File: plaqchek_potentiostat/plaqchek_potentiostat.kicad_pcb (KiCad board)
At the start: 4 copper layers, 46 x 59 mm, 63 parts, among them J1 Conn_01x03, J2 Conn_01x03, J3 Conn_01x02, SW2 SW_SPDT, U1 TL082, U3 TL082, U4 TL082, U5 TPS7A2050PDBVR, U6 MC79M05_TO252

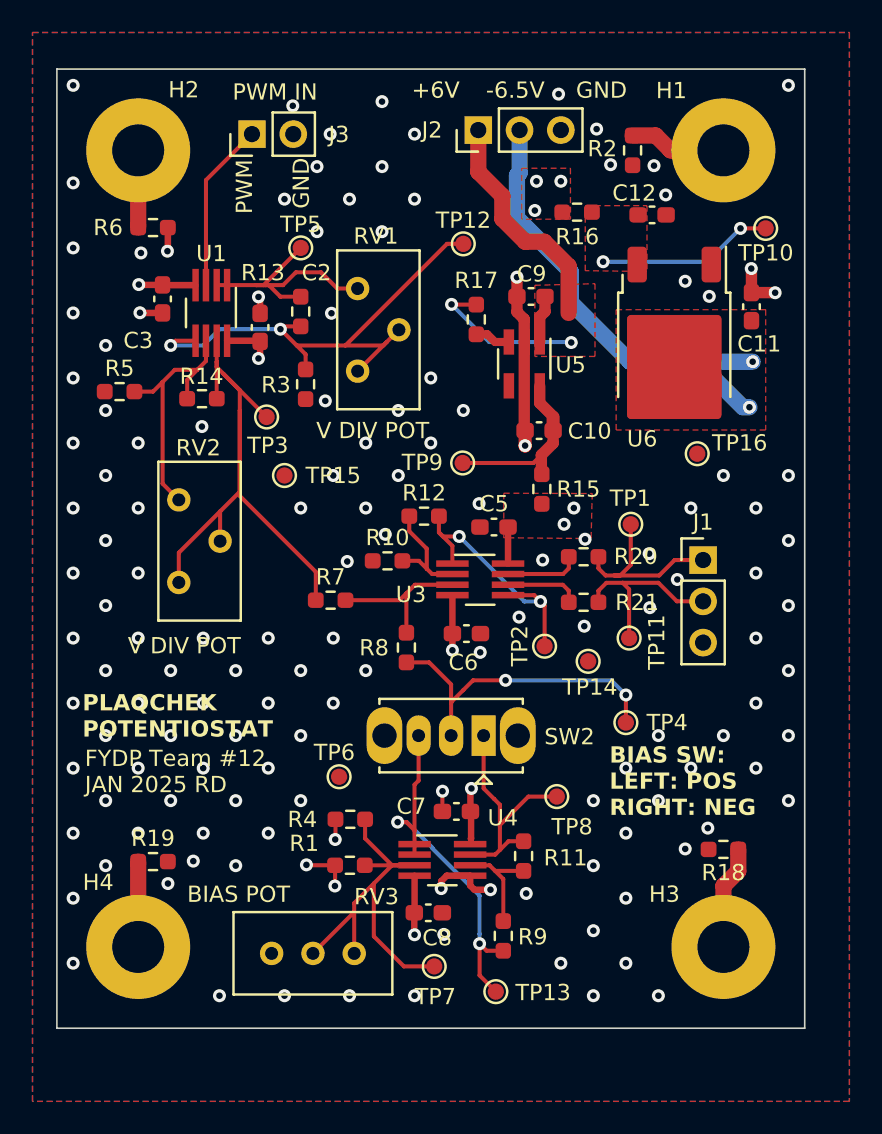
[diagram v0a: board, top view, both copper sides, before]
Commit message: finish all pcbs, generate gerber files
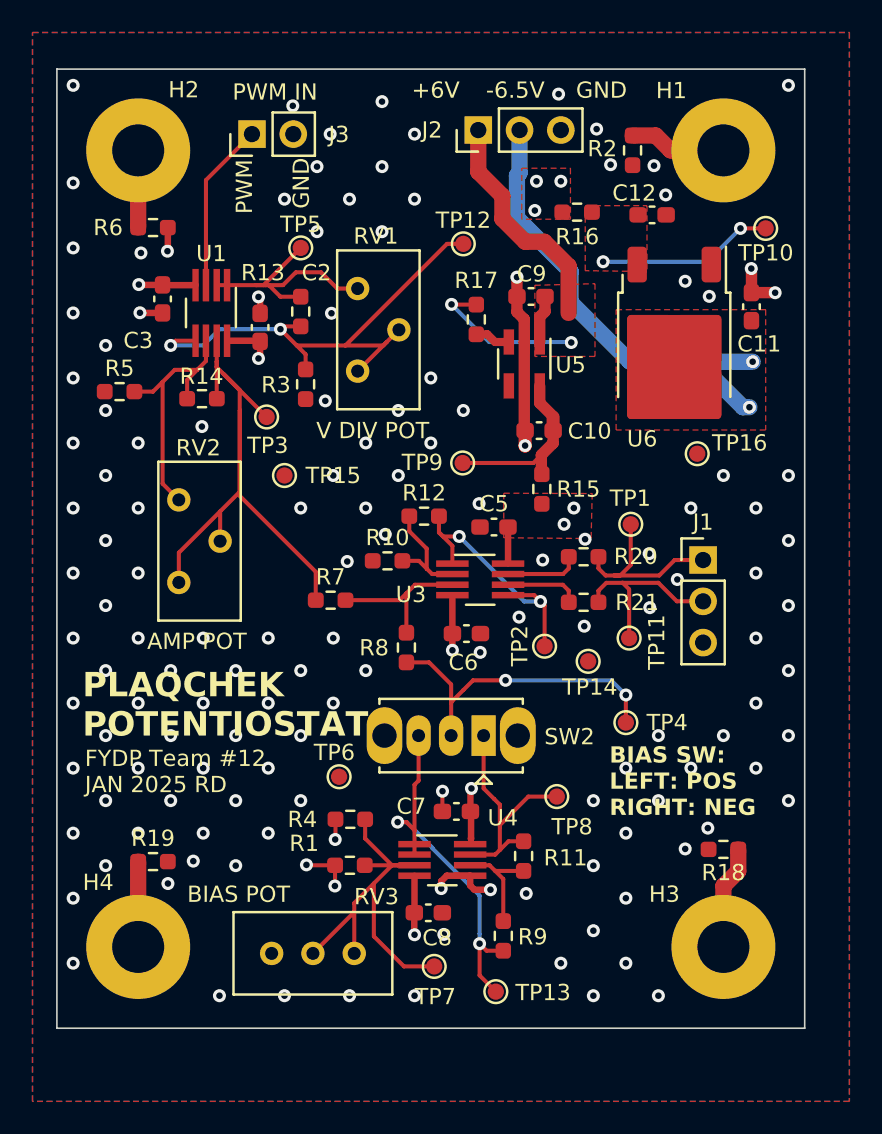
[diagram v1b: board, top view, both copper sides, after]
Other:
- board text added: "AMP POT"
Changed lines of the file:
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@@
       (outputformat 1)
       (mirror false)
-      (drillshape 1)
+      (drillshape 0)
       (scaleselection 1)
-      (outputdirectory "")
+      (outputdirectory "plaqchek_potentiostat_gerbers/")
     )
   )
@@
     (fp_line (start 4.11 2.7) (end 3.11 2.7)
       (stroke (width 0.1) (type solid)) (layer "F.Fab"))
-    (pad "1" smd roundrect (at -5.04 -2.28 270) (size 2.2 1.2) (layers "F.Cu" "F.Paste" "F.Mask") (roundrect_rratio 0.208333)
+    (pad "1" smd roundrect (at -5.04 -2.28 270) (size 2.2 1.2) (layers "F.Cu" "F.Paste" "F.Mask") (roundrect_rratio 0.2083333333)
       (net 1 "GND") (pinfunction "GND") (pintype "power_in"))
-    (pad "2" smd roundrect (at -0.415 -1.525 270) (size 3.05 2.75) (layers "F.Cu" "F.Paste") (roundrect_rratio 0.090909)
+    (pad "2" smd roundrect (at -0.415 -1.525 270) (size 3.05 2.75) (layers "F.Cu" "F.Paste") (roundrect_rratio 0.09090909091)
       (net 6 "-6V5") (pinfunction "VI") (pintype "power_in"))
-    (pad "2" smd roundrect (at -0.415 1.525 270) (size 3.05 2.75) (layers "F.Cu" "F.Paste") (roundrect_rratio 0.090909)
+    (pad "2" smd roundrect (at -0.415 1.525 270) (size 3.05 2.75) (layers "F.Cu" "F.Paste") (roundrect_rratio 0.09090909091)
       (net 6 "-6V5") (pinfunction "VI") (pintype "power_in"))
-    (pad "2" smd roundrect (at 1.26 0 270) (size 6.4 5.8) (layers "F.Cu" "F.Mask") (roundrect_rratio 0.043103)
+    (pad "2" smd roundrect (at 1.26 0 270) (size 6.4 5.8) (layers "F.Cu" "F.Mask") (roundrect_rratio 0.04310293103)
       (net 6 "-6V5") (pinfunction "VI") (pintype "power_in"))
-    (pad "2" smd roundrect (at 2.935 -1.525 270) (size 3.05 2.75) (layers "F.Cu" "F.Paste") (roundrect_rratio 0.090909)
+    (pad "2" smd roundrect (at 2.935 -1.525 270) (size 3.05 2.75) (layers "F.Cu" "F.Paste") (roundrect_rratio 0.09090909091)
       (net 6 "-6V5") (pinfunction "VI") (pintype "power_in"))
-    (pad "2" smd roundrect (at 2.935 1.525 270) (size 3.05 2.75) (layers "F.Cu" "F.Paste") (roundrect_rratio 0.090909)
+    (pad "2" smd roundrect (at 2.935 1.525 270) (size 3.05 2.75) (layers "F.Cu" "F.Paste") (roundrect_rratio 0.09090909091)
       (net 6 "-6V5") (pinfunction "VI") (pintype "power_in"))
-    (pad "3" smd roundrect (at -5.04 2.28 270) (size 2.2 1.2) (layers "F.Cu" "F.Paste" "F.Mask") (roundrect_rratio 0.208333)
+    (pad "3" smd roundrect (at -5.04 2.28 270) (size 2.2 1.2) (layers "F.Cu" "F.Paste" "F.Mask") (roundrect_rratio 0.2083333333)
       (net 7 "/-5V_R") (pinfunction "VO") (pintype "power_out"))
     (model "${KICAD6_3DMODEL_DIR}/Package_TO_SOT_SMD.3dshapes/TO-252-2.wrl"
@@
     (effects (font (size 1 1) (thickness 0.153) bold) (justify left bottom))
   )
-  (gr_text "V DIV POT" (at 148.36 123.06) (layer "F.SilkS" knockout)
+  (gr_text "AMP POT" (at 149.55 122.79) (layer "F.SilkS" knockout)
     (effects (font (size 1 1) (thickness 0.153)) (justify left bottom))
   )
@@
   )
   (gr_text "PLAQCHEK\nPOTENTIOSTAT" (at 145.57 128.18) (layer "F.SilkS")
-    (effects (font (size 1 1) (thickness 0.153) bold) (justify left bottom))
+    (effects (font (size 1.5 1.5) (thickness 0.3) bold) (justify left bottom))
   )
   (gr_text "-6.5V\n" (at 172.2 88.3) (layer "F.SilkS" knockout)
